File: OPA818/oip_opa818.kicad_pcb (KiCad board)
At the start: 2 copper layers, 25 x 25 mm, 32 parts, among them J101 Conn_Coaxial, J102 Conn_01x03, U101 LT3042xMSE, U102 LT3093xMSE, U103 OPA818IDRGx, U104 BUF602xDBV

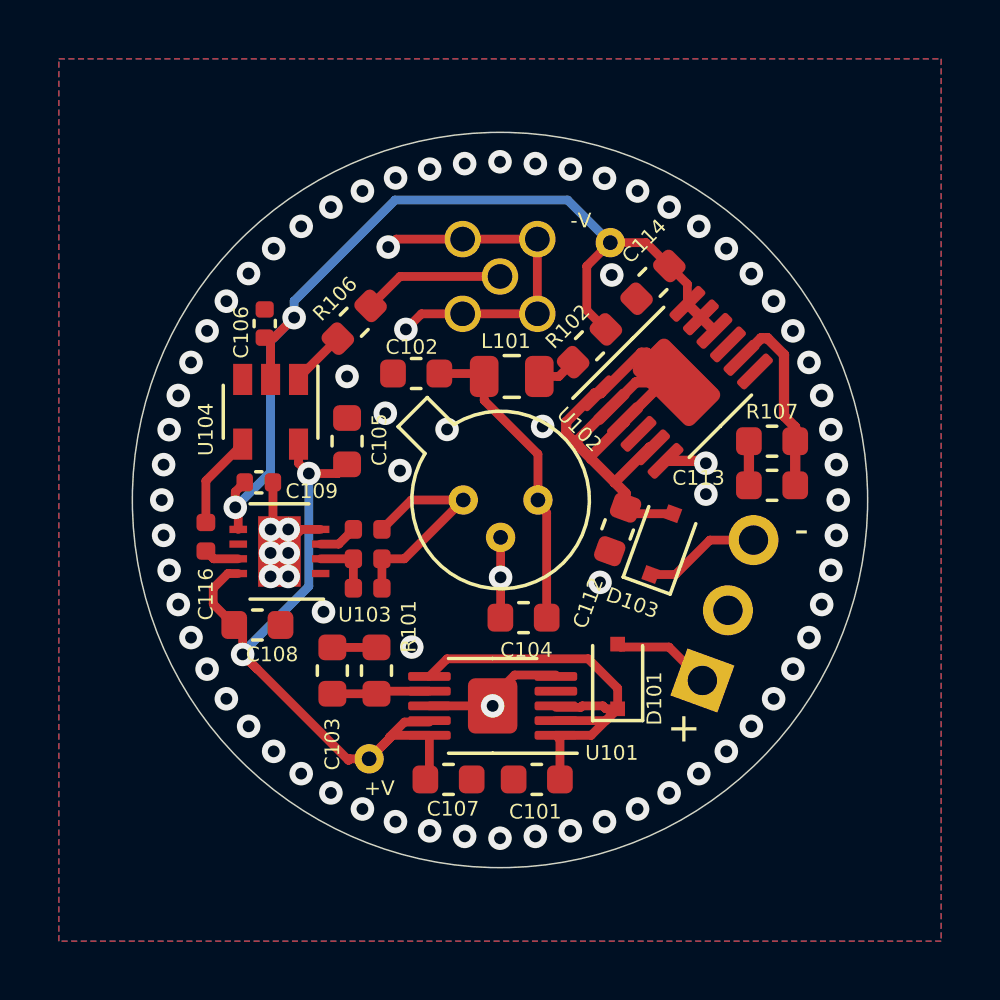
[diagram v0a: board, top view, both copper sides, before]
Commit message: v6
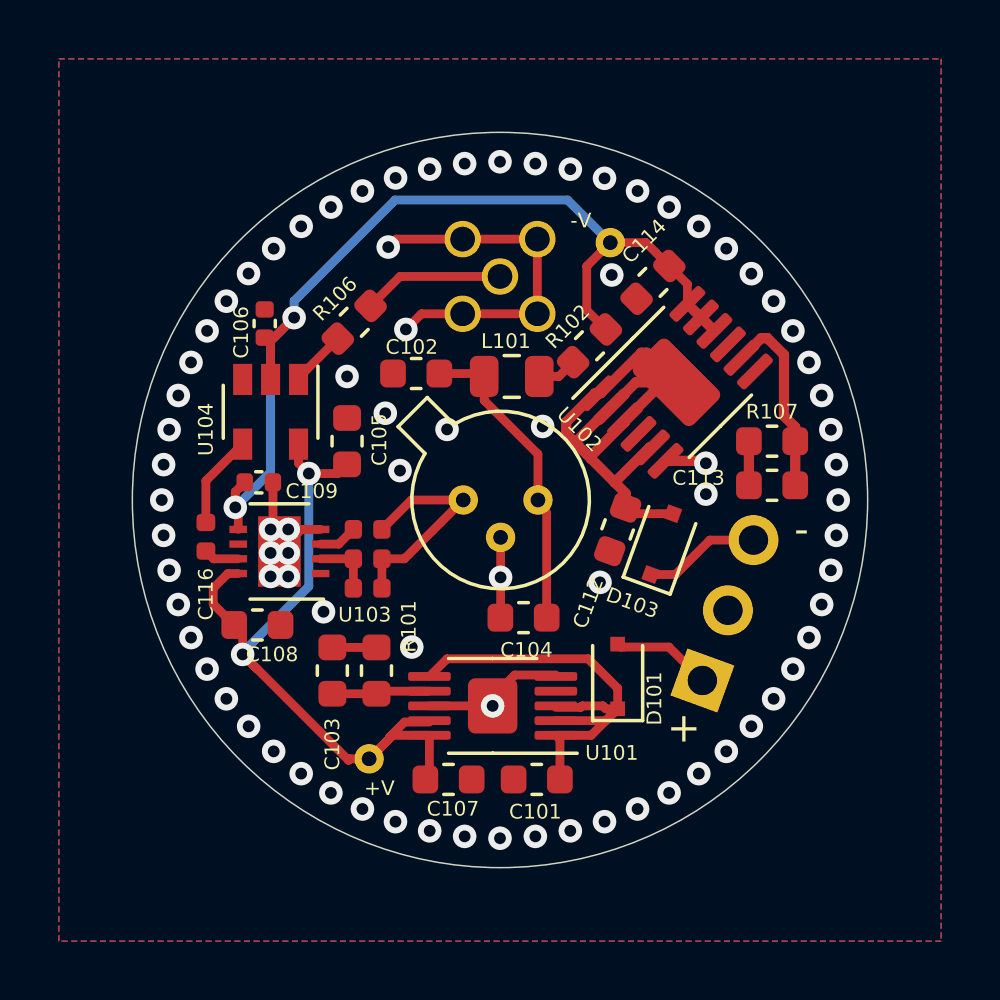
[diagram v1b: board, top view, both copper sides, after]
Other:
- net class Default removed
- net class PWR removed
